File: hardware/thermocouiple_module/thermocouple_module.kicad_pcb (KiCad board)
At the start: 2 copper layers, 19 x 27.9 mm, 12 parts, among them P1 CONN_2, P2 CONN_1, P3 CONN_4, P4 CONN_2, P5 CONN_1, P6 CONN_1, P7 CONN_2, U5 MAX31855KASA

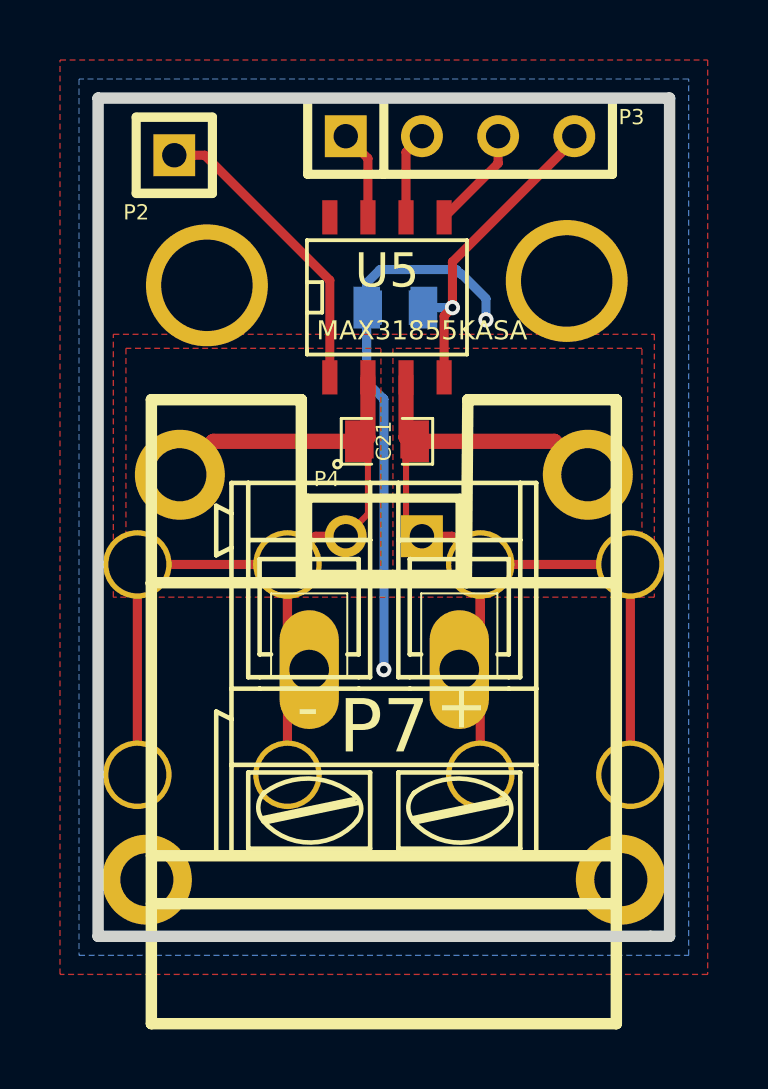
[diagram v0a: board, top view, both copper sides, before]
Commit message: update pcb files
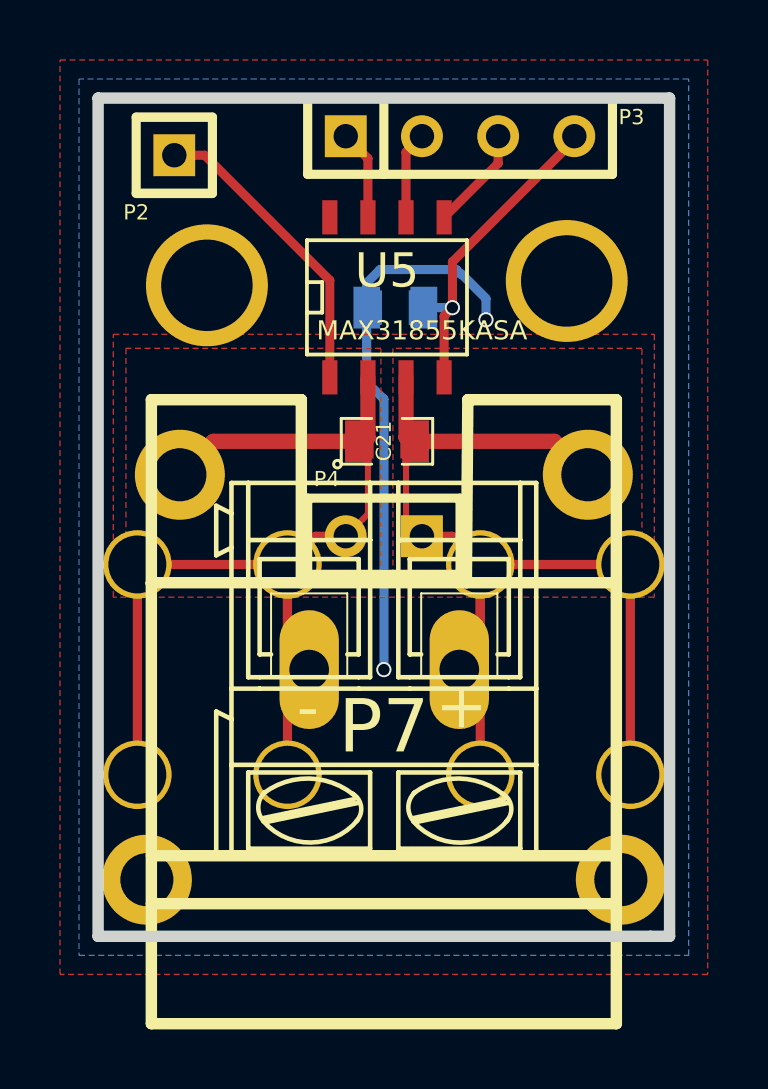
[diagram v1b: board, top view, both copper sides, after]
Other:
- net class Default removed
